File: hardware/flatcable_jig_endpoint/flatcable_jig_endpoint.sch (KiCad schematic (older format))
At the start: 9 parts

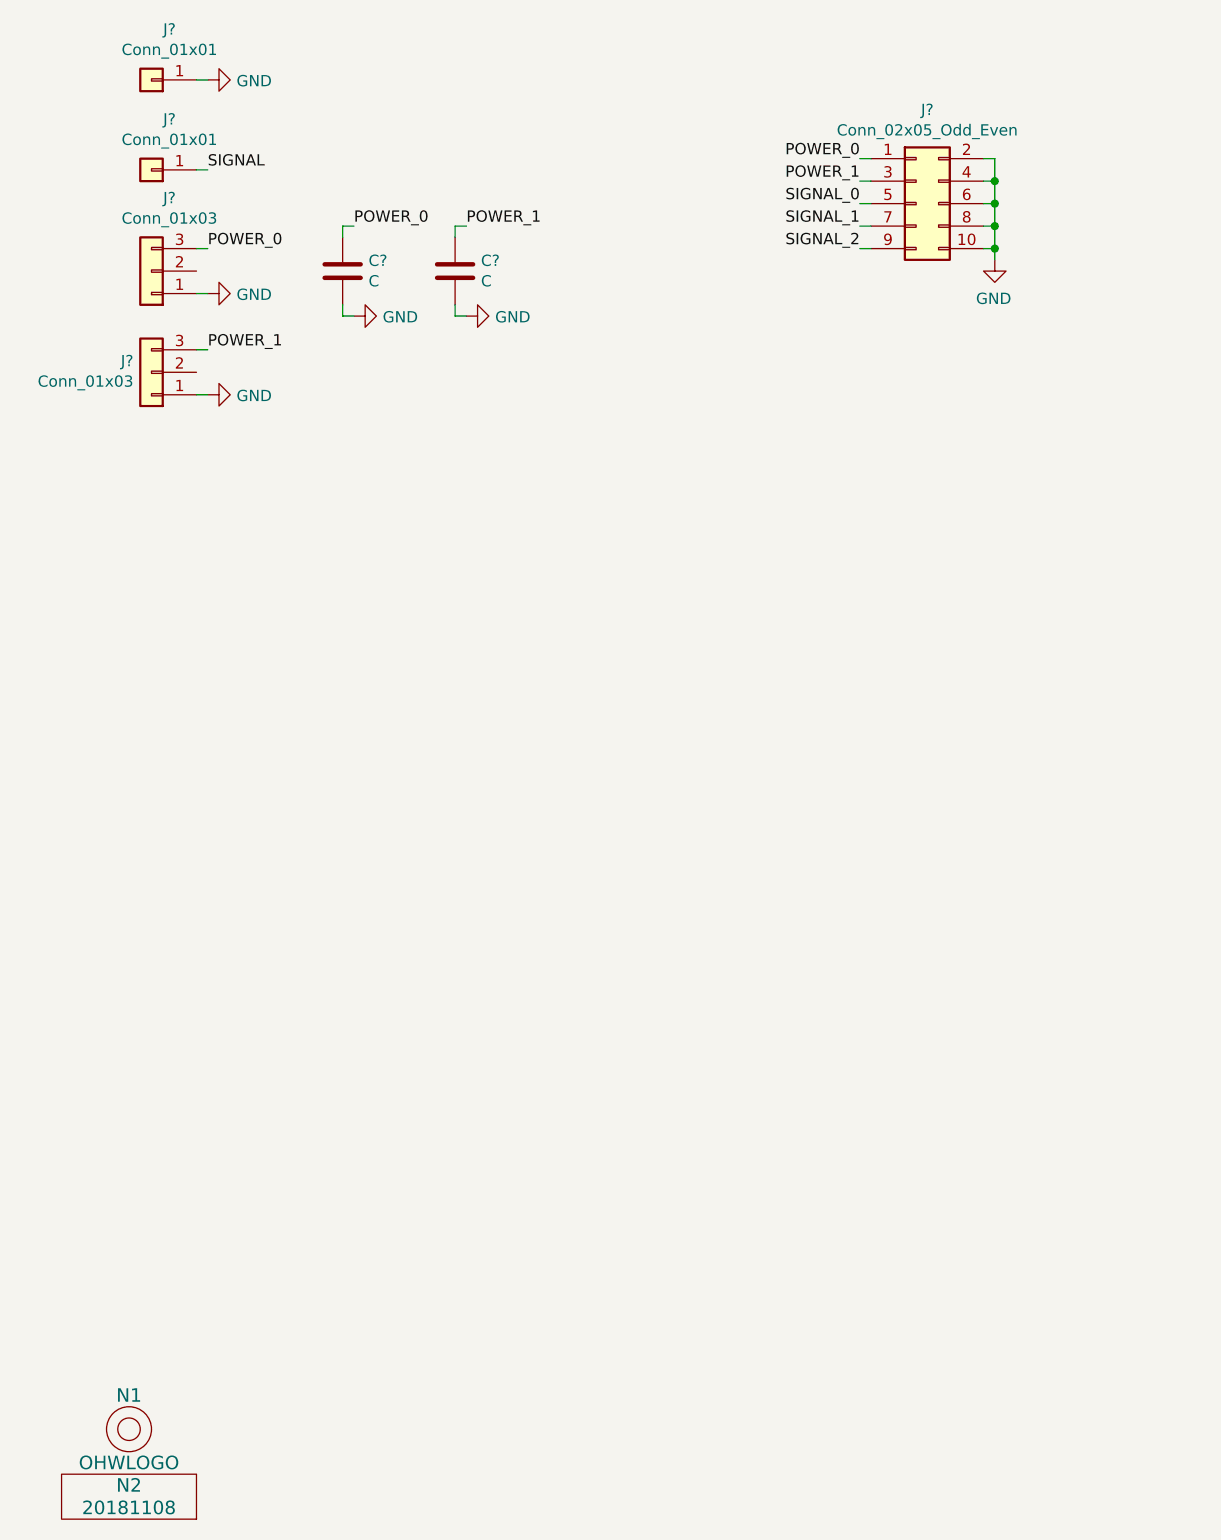
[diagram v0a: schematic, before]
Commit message: started layout, still need to add the endpad connections
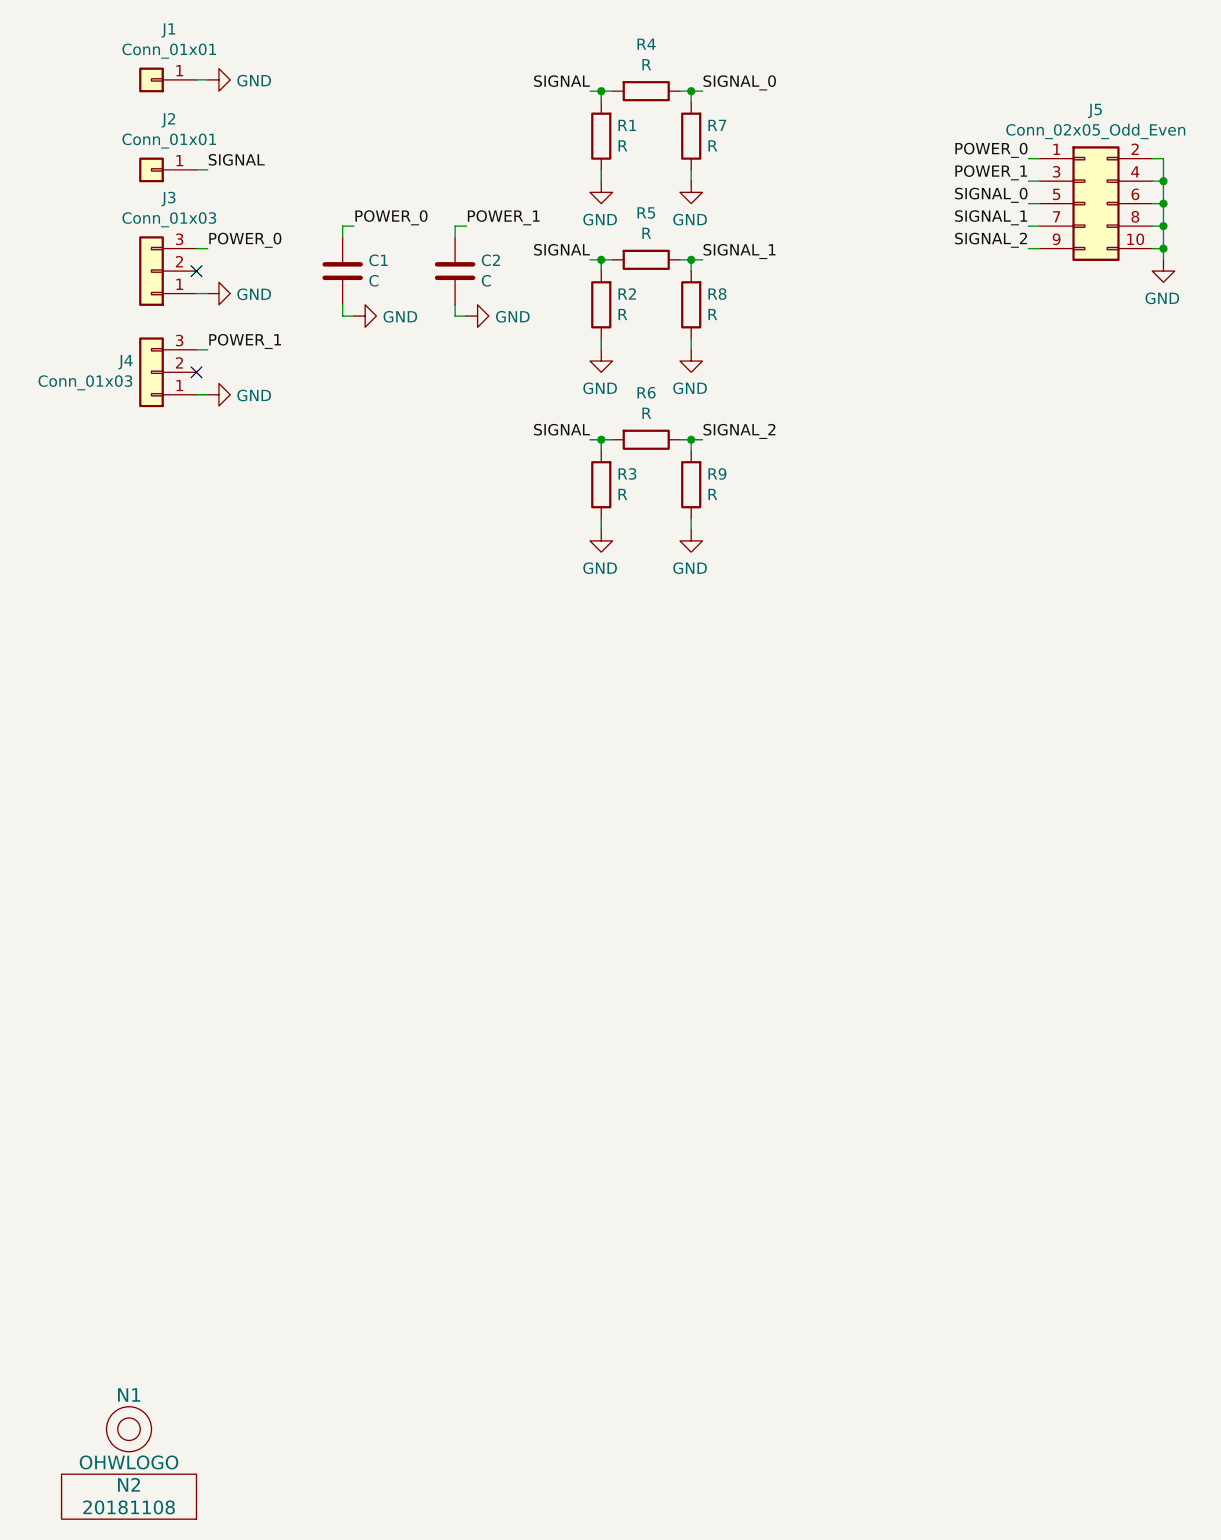
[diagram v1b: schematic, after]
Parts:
- added R1, R2, R3, R4, R5, R6, R7, R8, R9: R, SquantorRcl:R_0603_hand, symbol Device:R
- J3, J4: renamed from J?; footprint (none) -> Connector_Molex:Molex_KK-254_AE-6410-03A_1x03_P2.54mm_Vertical
- J5: renamed from J?; footprint (none) -> SquantorConnectors:Header-0254-2X05-H010
- gave numbers to parts that had none: 4
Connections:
- net GND: now also R1.1, R2.1, R3.1, R7.1, R8.1, R9.1
- net SIGNAL: now also R1.2, R2.2, R3.2, R4.2, R5.2, R6.2
- net SIGNAL_0: now also R4.1, R7.2
- net SIGNAL_1: now also R5.1, R8.2
- net SIGNAL_2: now also R6.1, R9.2
- no-connect marks 0 -> 2
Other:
- moved on the sheet: J5
